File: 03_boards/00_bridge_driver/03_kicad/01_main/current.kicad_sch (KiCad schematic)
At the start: 24 parts, among them U10 REF3020, U11 INA241A2xD, U12 AMC1311, U13 AMC1311, U16 INA241A2xD

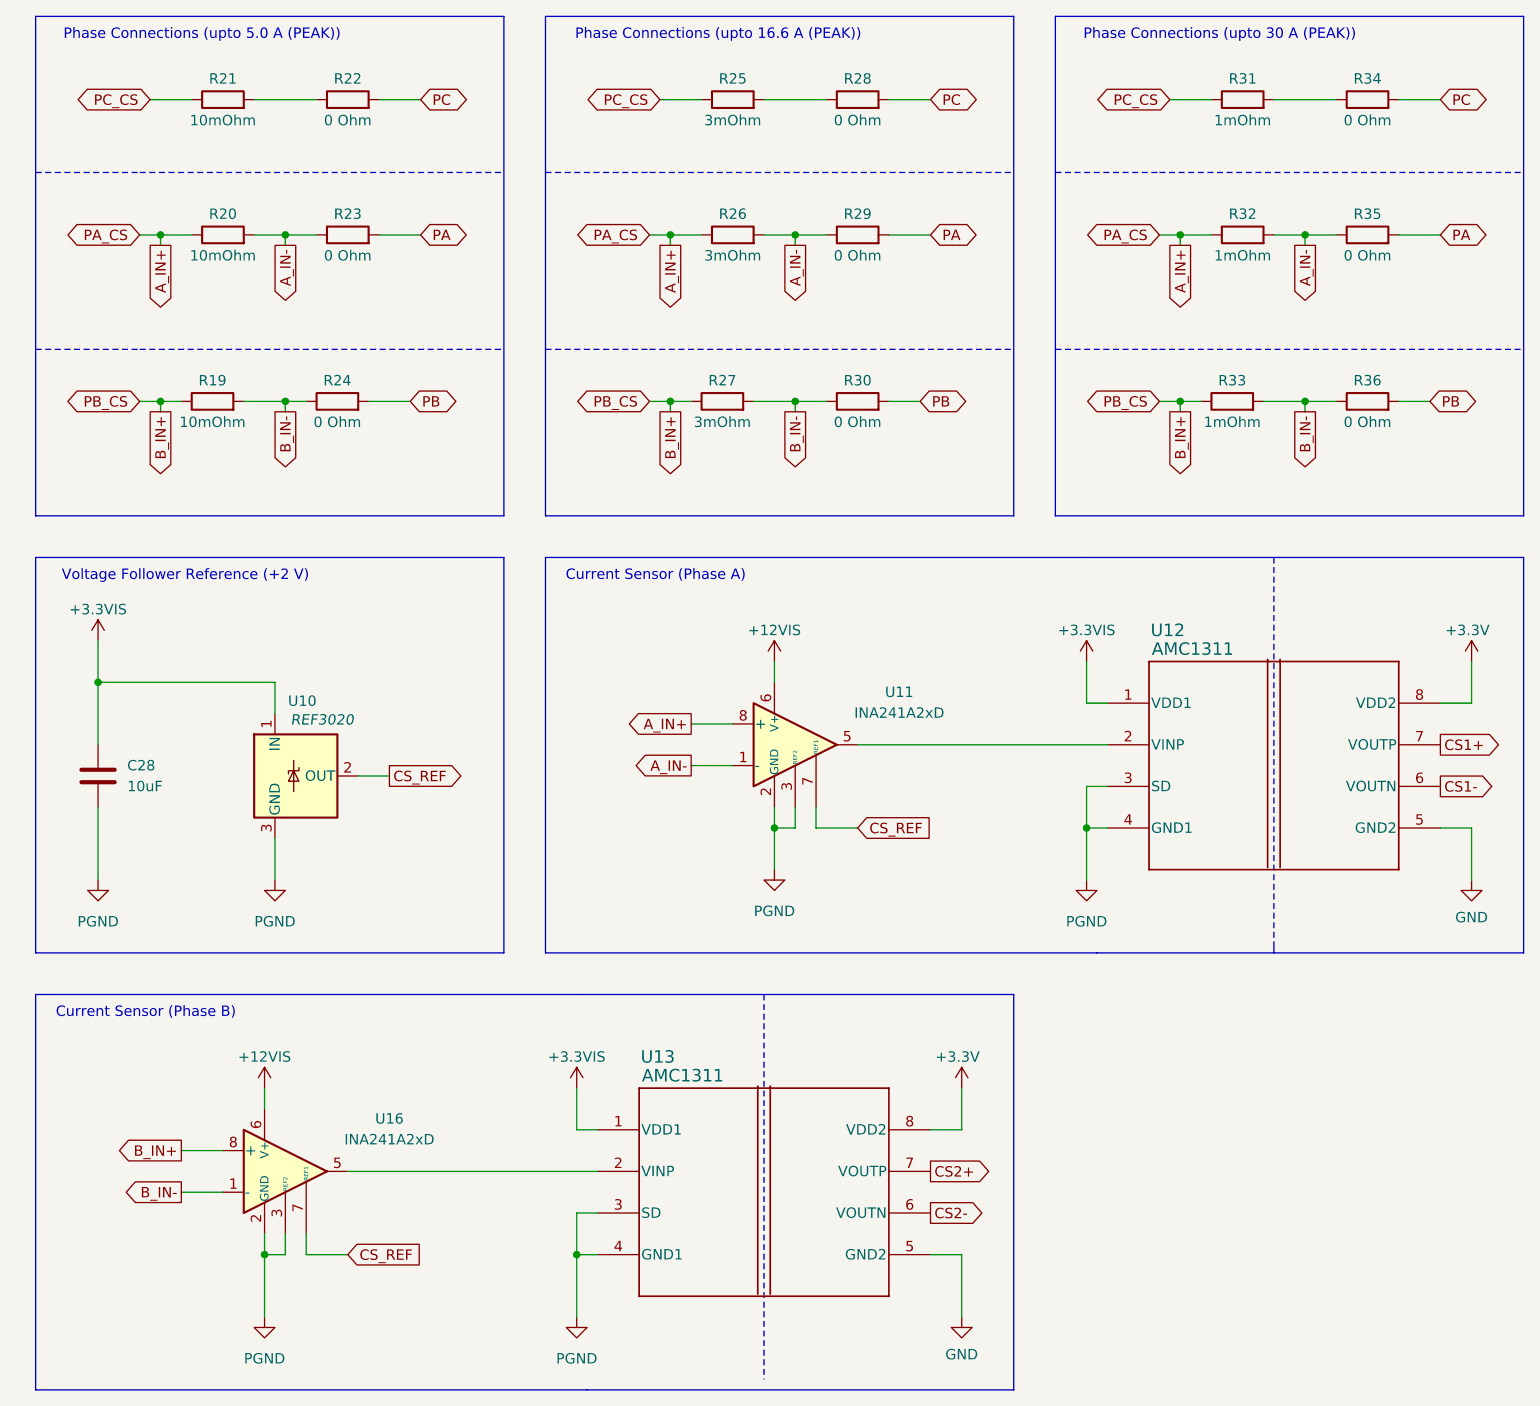
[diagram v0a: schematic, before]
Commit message: Initial PCB modelling work
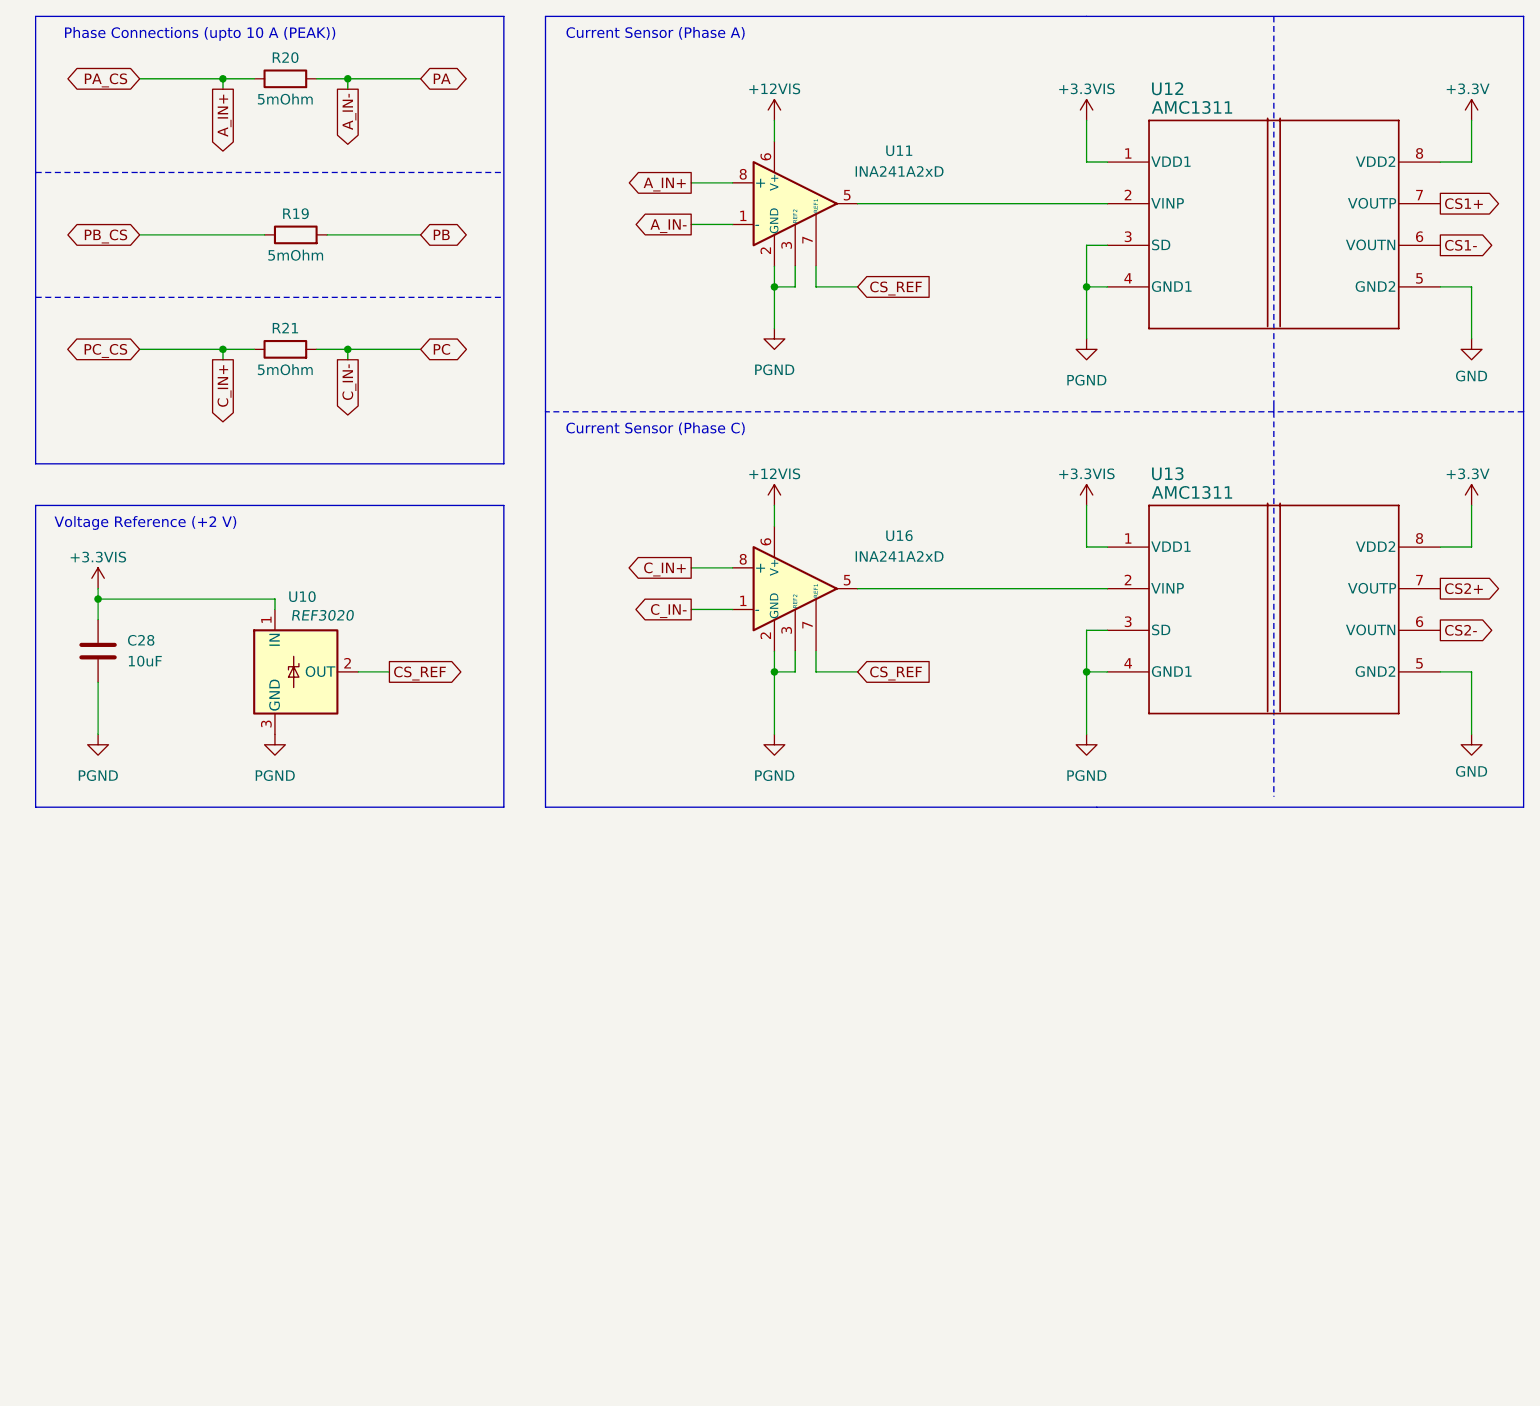
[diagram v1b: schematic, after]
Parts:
- removed R22, R23, R24, R28, R29, R30, R34, R35, R36: 0 Ohm, Resistor_SMD:R_2512_6332Metric, symbol Device:R
- removed R25, R26, R27: 3mOhm, Resistor_SMD:R_2512_6332Metric, symbol Device:R
- removed R31, R32, R33: 1mOhm, Resistor_SMD:R_2512_6332Metric, symbol Device:R
- R19, R20, R21: value 10mOhm -> 5mOhm
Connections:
- net PC_CS is gone; now on net C_IN+: R21.1
- net PB: now also R19.2
- net C_IN-: now reaches R21.2
- net C_IN-: now also U16.1 (-)
- net B_IN+ renamed C_IN+
- net C_IN+: no longer R19.1
- removed net B_IN-: R19.2, U16.1 (-)
- new net PB_CS: R19.1
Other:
- note added: "Current Sensor (Phase C)"
- note added: "Phase Connections (upto 10 A (PEAK))"
- note added: "Voltage Reference (+2 V)"
- note removed: "Current Sensor (Phase B)"
- note removed: "Phase Connections (upto 16.6 A (PEAK))"
- note removed: "Phase Connections (upto 30 A (PEAK))"
- note removed: "Phase Connections (upto 5.0 A (PEAK))"
- note removed: "Voltage Follower Reference (+2 V)"
- moved on the sheet: C28, R19, R20, R21, U10, U11, U12, U13, U16
